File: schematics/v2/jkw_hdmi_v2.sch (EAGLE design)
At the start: 32 parts, among them J1 2X20-CHIP-HEADERS, J2 T_MOLEX_45171, U1 DS2431P

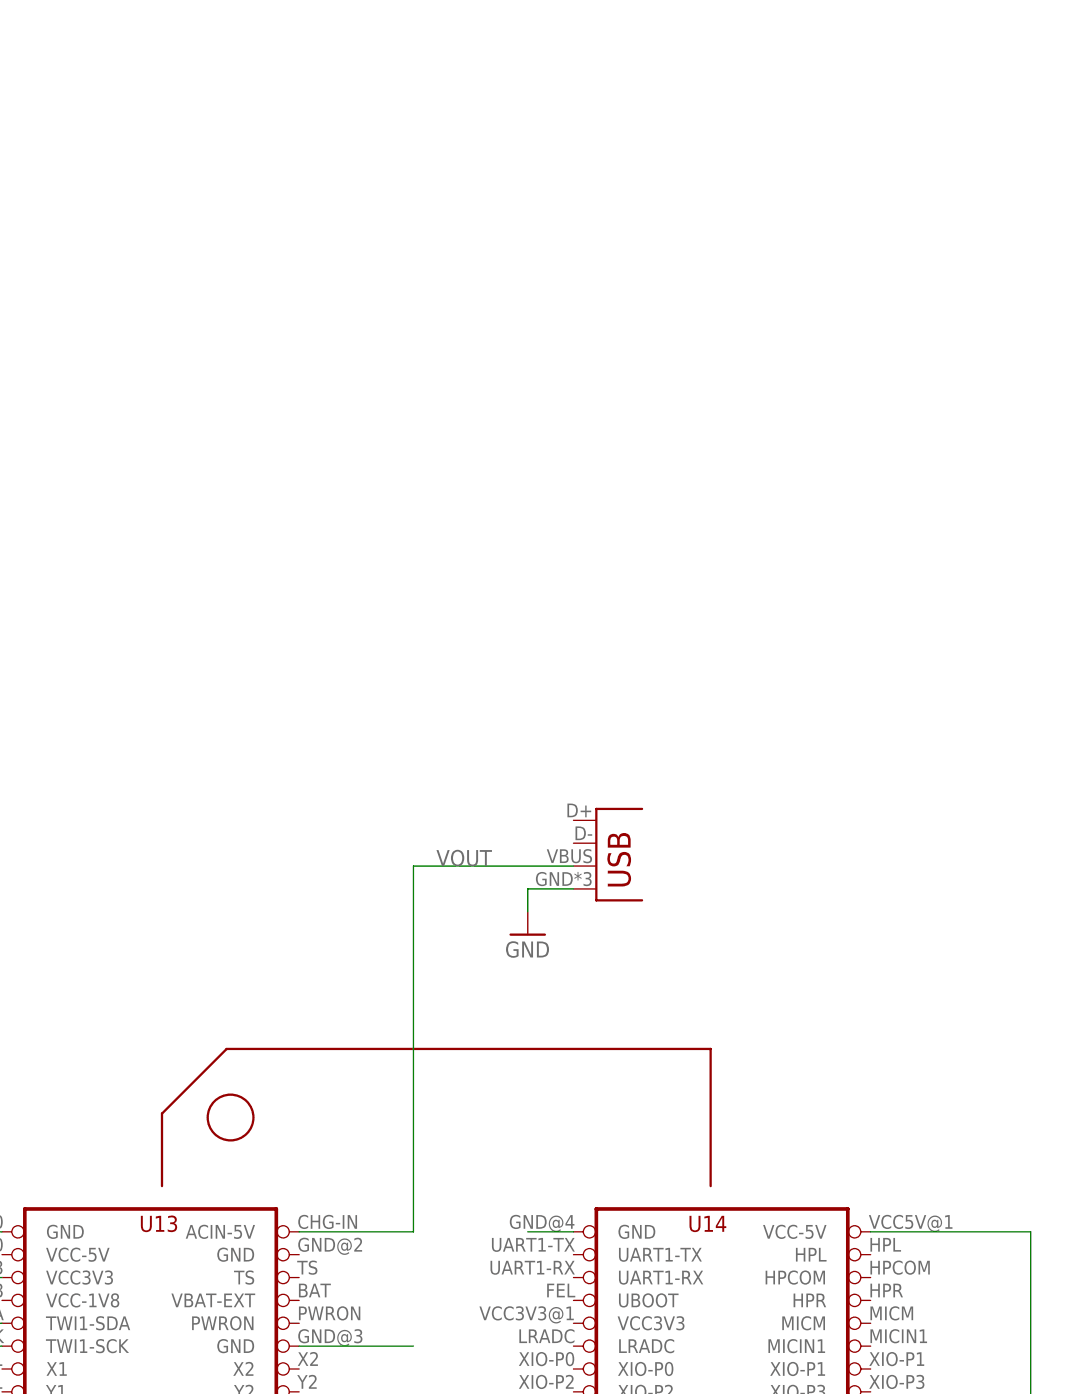
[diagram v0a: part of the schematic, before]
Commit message: added v2 with DCDC
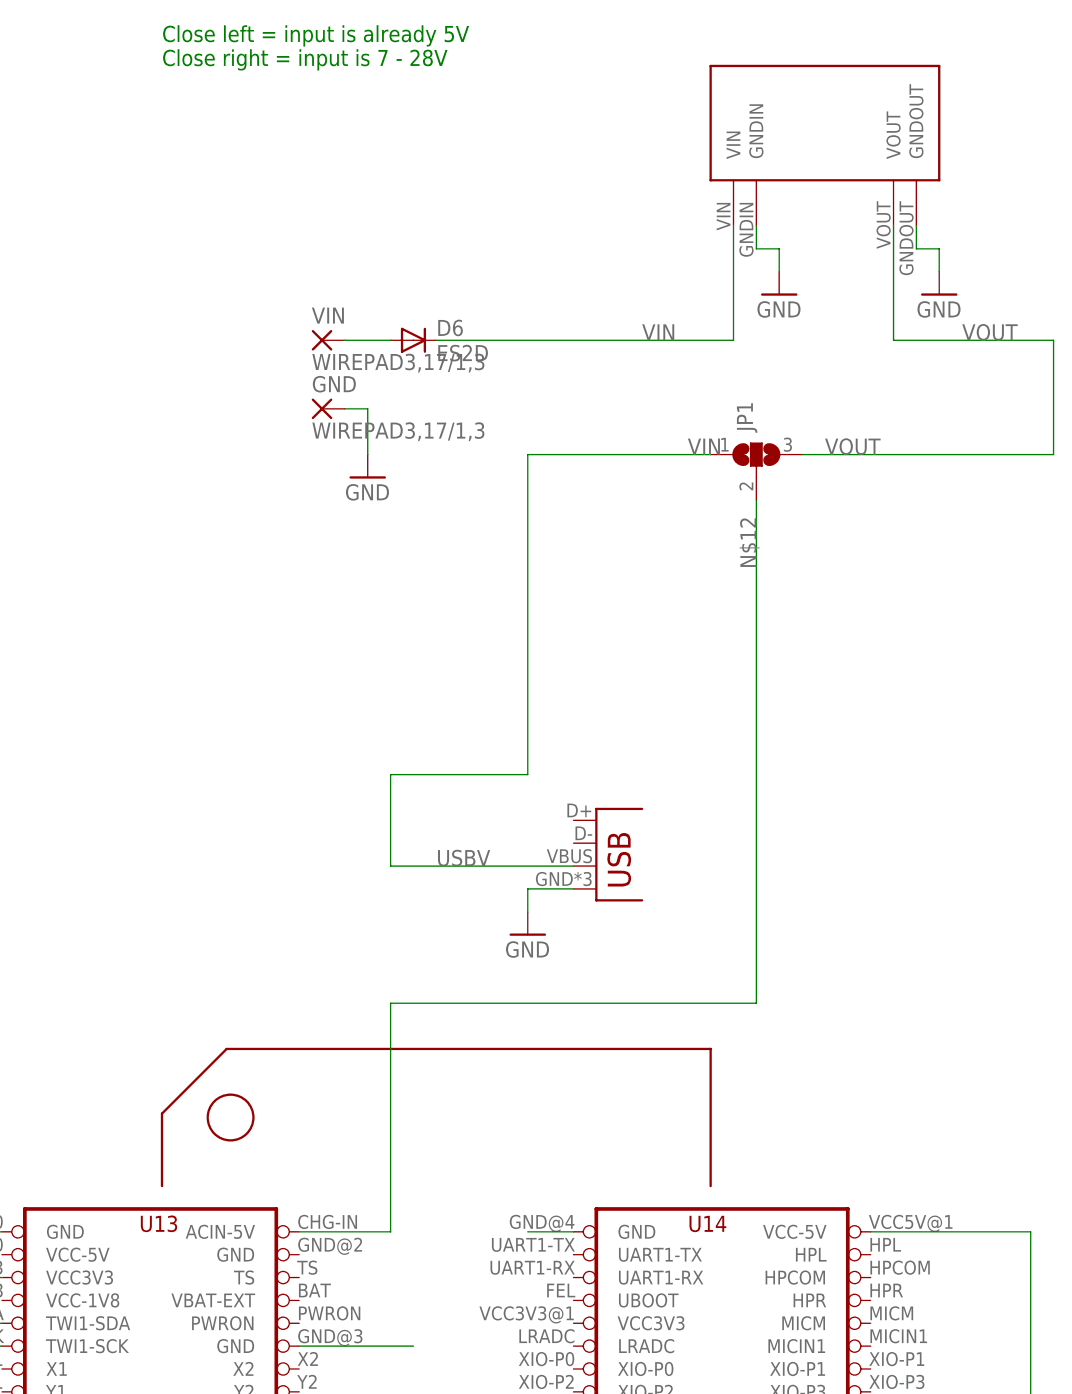
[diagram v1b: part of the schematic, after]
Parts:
- added D6: ES2D, diode:ES2D
- added GND, VIN: WIREPAD3,17/1,3, wirepad:WIREPAD3,17/1,3
- added JP1: (no value), jumper:SJ2W
- added U$9: MP1584EN, power_supply:MP1584EN
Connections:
- new net N$12: J1.ACIN-5V, JP1.2
- new net N$65: D6.A, VIN.P
- new net USBV: JP1.1, POWER_USB.VBUS
- new net VIN: D6.C, U$9.VIN
- net GND: now also GND.P, U$9.GNDIN, U$9.GNDOUT
- net VOUT: now also JP1.3, U$9.VOUT; no longer J1.ACIN-5V, POWER_USB.VBUS
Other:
- note added: "Close left = input is already 5V Close right = input is 7 - 28V"
- note added: "Power supply 1"
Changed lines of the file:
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@@
 <layers>
 <layer number="1" name="Top" color="4" fill="1" visible="no" active="no"/>
+<layer number="2" name="Route2" color="1" fill="3" visible="no" active="no"/>
+<layer number="3" name="Route3" color="4" fill="3" visible="no" active="no"/>
+<layer number="14" name="Route14" color="1" fill="6" visible="no" active="no"/>
+<layer number="15" name="Route15" color="4" fill="6" visible="no" active="no"/>
 <layer number="16" name="Bottom" color="1" fill="1" visible="no" active="no"/>
 <layer number="17" name="Pads" color="2" fill="1" visible="no" active="no"/>
@@
 <part name="POWER_USB" library="Spark" deviceset="USB" device="USB-MICROB-SMT-DIP"/>
 <part name="GND23" library="supply1" deviceset="GND" device=""/>
+<part name="U$9" library="power_supply" deviceset="MP1584EN" device=""/>
+<part name="JP1" library="jumper" deviceset="SJ2W" device=""/>
+<part name="GND24" library="supply1" deviceset="GND" device=""/>
+<part name="GND25" library="supply1" deviceset="GND" device=""/>
+<part name="VIN" library="wirepad" deviceset="WIREPAD" device="3,17/1,3"/>
+<part name="GND" library="wirepad" deviceset="WIREPAD" device="3,17/1,3"/>
+<part name="GND26" library="supply1" deviceset="GND" device=""/>
+<part name="D6" library="diode" deviceset="ES2D" device=""/>
 </parts>
 <sheets>
@@
 <text x="7.62" y="78.74" size="1.778" layer="91">i2c adr = 7F</text>
 <text x="7.62" y="76.2" size="1.778" layer="91">i2c adr = 7F</text>
+<text x="175.26" y="226.06" size="1.778" layer="91">Close left = input is already 5V
+Close right = input is 7 - 28V</text>
+<text x="228.6" y="228.6" size="2.54" layer="103">Power supply 1</text>
 </plain>
 <instances>
@@
 <instance part="POWER_USB" gate="G$1" x="223.52" y="134.62"/>
 <instance part="GND23" gate="1" x="215.9" y="129.54"/>
+<instance part="U$9" gate="G$1" x="236.22" y="213.36"/>
+<instance part="JP1" gate="G$1" x="241.3" y="182.88" rot="R90"/>
+<instance part="GND24" gate="1" x="243.84" y="200.66"/>
+<instance part="GND25" gate="1" x="261.62" y="200.66"/>
+<instance part="VIN" gate="G$1" x="193.04" y="195.58"/>
+<instance part="GND" gate="G$1" x="193.04" y="187.96"/>
+<instance part="GND26" gate="1" x="198.12" y="180.34"/>
+<instance part="D6" gate="G$1" x="203.2" y="195.58"/>
 </instances>
 <busses>
@@
 <wire x1="215.9" y1="134.62" x2="215.9" y2="132.08" width="0.1524" layer="91"/>
 </segment>
+<segment>
+<pinref part="U$9" gate="G$1" pin="GNDIN"/>
+<wire x1="241.3" y1="208.28" x2="241.3" y2="205.74" width="0.1524" layer="91"/>
+<pinref part="GND24" gate="1" pin="GND"/>
+<wire x1="241.3" y1="205.74" x2="243.84" y2="205.74" width="0.1524" layer="91"/>
+<wire x1="243.84" y1="205.74" x2="243.84" y2="203.2" width="0.1524" layer="91"/>
+</segment>
+<segment>
+<pinref part="U$9" gate="G$1" pin="GNDOUT"/>
+<wire x1="259.08" y1="208.28" x2="259.08" y2="205.74" width="0.1524" layer="91"/>
+<pinref part="GND25" gate="1" pin="GND"/>
+<wire x1="259.08" y1="205.74" x2="261.62" y2="205.74" width="0.1524" layer="91"/>
+<wire x1="261.62" y1="205.74" x2="261.62" y2="203.2" width="0.1524" layer="91"/>
+</segment>
+<segment>
+<pinref part="GND" gate="G$1" pin="P"/>
+<pinref part="GND26" gate="1" pin="GND"/>
+<wire x1="195.58" y1="187.96" x2="198.12" y2="187.96" width="0.1524" layer="91"/>
+<wire x1="198.12" y1="187.96" x2="198.12" y2="182.88" width="0.1524" layer="91"/>
+</segment>
 </net>
 <net name="LCD-D3" class="0">
@@
 <net name="VOUT" class="0">
 <segment>
+<pinref part="JP1" gate="G$1" pin="3"/>
+<label x="248.92" y="182.88" size="1.778" layer="95"/>
+<wire x1="246.38" y1="182.88" x2="274.32" y2="182.88" width="0.1524" layer="91"/>
+<wire x1="274.32" y1="182.88" x2="274.32" y2="195.58" width="0.1524" layer="91"/>
+<pinref part="U$9" gate="G$1" pin="VOUT"/>
+<wire x1="256.54" y1="208.28" x2="256.54" y2="195.58" width="0.1524" layer="91"/>
+<wire x1="256.54" y1="195.58" x2="274.32" y2="195.58" width="0.1524" layer="91"/>
+<label x="264.16" y="195.58" size="1.778" layer="95"/>
+</segment>
+</net>
+<net name="VIN" class="0">
+<segment>
+<label x="233.68" y="182.88" size="1.778" layer="95"/>
+<pinref part="U$9" gate="G$1" pin="VIN"/>
+<wire x1="238.76" y1="208.28" x2="238.76" y2="195.58" width="0.1524" layer="91"/>
+<wire x1="238.76" y1="195.58" x2="205.74" y2="195.58" width="0.1524" layer="91"/>
+<label x="228.6" y="195.58" size="1.778" layer="95"/>
+<pinref part="D6" gate="G$1" pin="C"/>
+</segment>
+</net>
+<net name="N$65" class="0">
+<segment>
+<pinref part="VIN" gate="G$1" pin="P"/>
+<wire x1="195.58" y1="195.58" x2="200.66" y2="195.58" width="0.1524" layer="91"/>
+<pinref part="D6" gate="G$1" pin="A"/>
+</segment>
+</net>
+<net name="N$12" class="0">
+<segment>
+<pinref part="J1" gate="G$1" pin="ACIN-5V"/>
+<wire x1="190.5" y1="96.52" x2="200.66" y2="96.52" width="0.1524" layer="91"/>
+<wire x1="200.66" y1="96.52" x2="200.66" y2="121.92" width="0.1524" layer="91"/>
+<pinref part="JP1" gate="G$1" pin="2"/>
+<label x="241.3" y="170.18" size="1.778" layer="95" rot="R90"/>
+<wire x1="200.66" y1="121.92" x2="241.3" y2="121.92" width="0.1524" layer="91"/>
+<wire x1="241.3" y1="121.92" x2="241.3" y2="177.8" width="0.1524" layer="91"/>
+</segment>
+</net>
+<net name="USBV" class="0">
+<segment>
 <pinref part="POWER_USB" gate="G$1" pin="VBUS"/>
-<wire x1="220.98" y1="137.16" x2="203.2" y2="137.16" width="0.1524" layer="91"/>
+<wire x1="220.98" y1="137.16" x2="200.66" y2="137.16" width="0.1524" layer="91"/>
 <label x="205.74" y="137.16" size="1.778" layer="95"/>
-<pinref part="J1" gate="G$1" pin="ACIN-5V"/>
-<wire x1="190.5" y1="96.52" x2="203.2" y2="96.52" width="0.1524" layer="91"/>
-<wire x1="203.2" y1="137.16" x2="203.2" y2="96.52" width="0.1524" layer="91"/>
+<wire x1="200.66" y1="137.16" x2="200.66" y2="147.32" width="0.1524" layer="91"/>
+<wire x1="215.9" y1="147.32" x2="215.9" y2="182.88" width="0.1524" layer="91"/>
+<pinref part="JP1" gate="G$1" pin="1"/>
+<wire x1="215.9" y1="182.88" x2="236.22" y2="182.88" width="0.1524" layer="91"/>
+<wire x1="200.66" y1="147.32" x2="215.9" y2="147.32" width="0.1524" layer="91"/>
 </segment>
 </net>
@@
 </schematic>
 </drawing>
+<compatibility>
+<note version="6.3" minversion="6.2.2" severity="warning">
+Since Version 6.2.2 text objects can contain more than one line,
+which will not be processed correctly with this version.
+</note>
+</compatibility>
 </eagle>
